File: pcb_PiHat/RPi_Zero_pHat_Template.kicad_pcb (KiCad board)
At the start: 2 copper layers, 65 x 30 mm, 9 parts, among them J1 RPi_GPIO, J2 Isolated_ISP, J3 Isolated_ISP, J4 Conn_Relay, J5 Conn_Relay

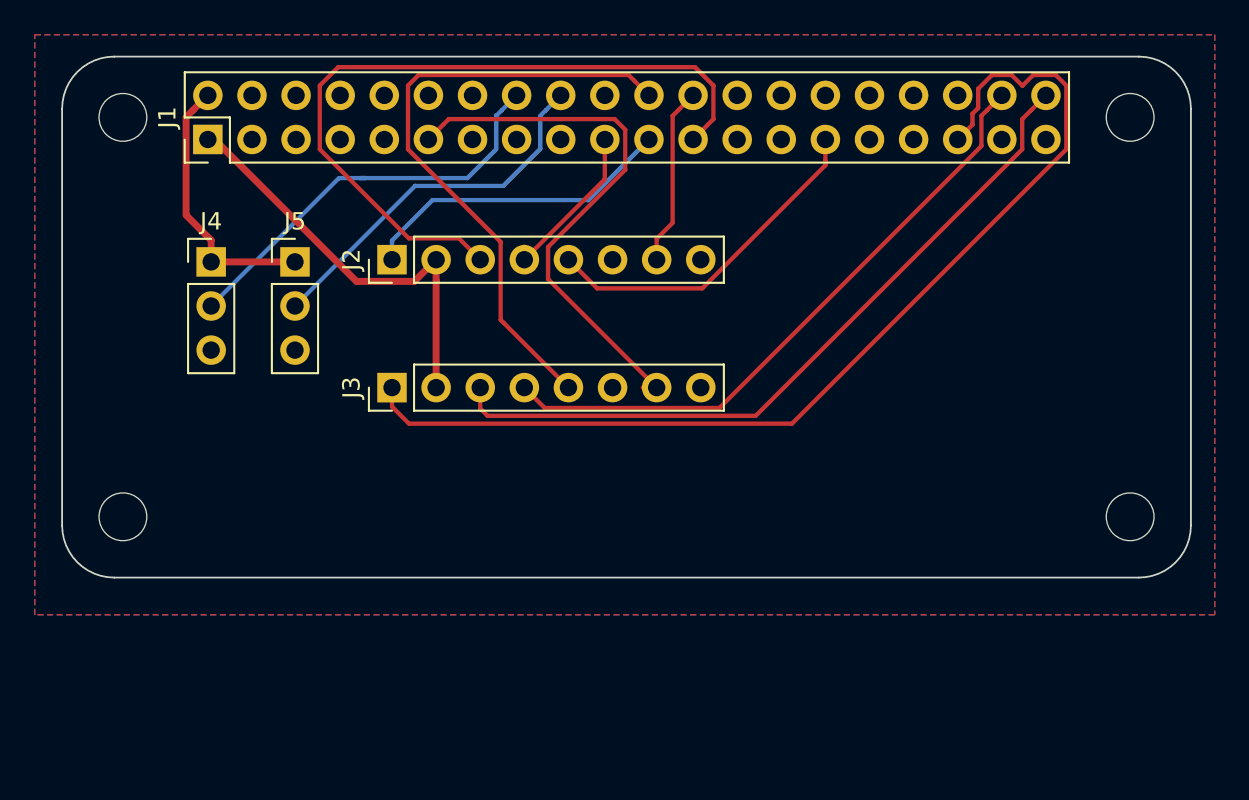
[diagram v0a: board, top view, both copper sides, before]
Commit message: raspi hat toteutettu versio
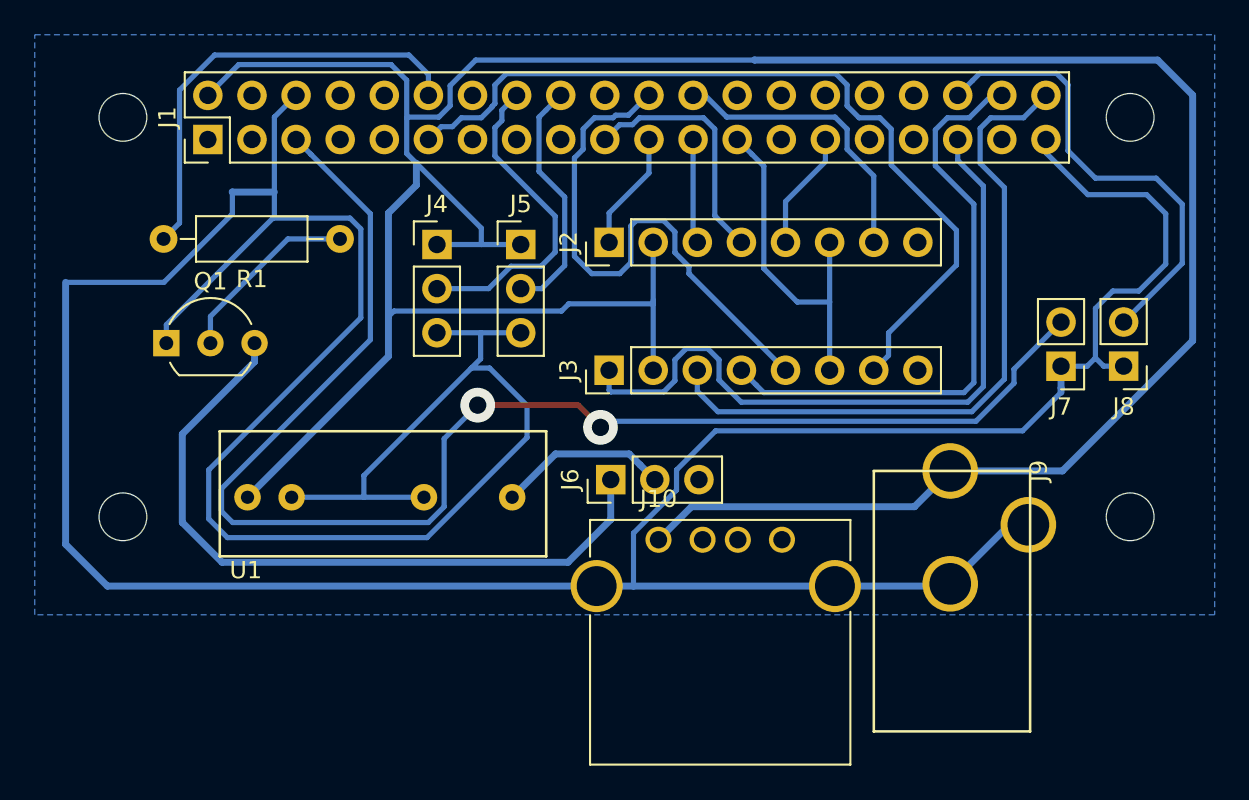
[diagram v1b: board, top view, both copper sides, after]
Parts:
- added J10: USB_A, Connectors:USB_A, F.Cu at (46.8, 52.3)
- added J6: Conn_01x03, Pin_Headers:Pin_Header_Straight_1x03_Pitch2.54mm, F.Cu at (44.1, 48.9)
- added J7: Conn_switch, Pin_Headers:Pin_Header_Straight_1x02_Pitch2.54mm, F.Cu at (70.0, 42.3)
- added J8: Conn_switch, Pin_Headers:Pin_Header_Straight_1x02_Pitch2.54mm, F.Cu at (73.6, 42.3)
- added J9: 5V_in, 5V_power:5V_power, F.Cu at (63.6, 48.4)
- added Q1: Q_NPN_EBC, TO_SOT_Packages_THT:TO-92_Inline_Wide, F.Cu at (18.5, 41.0)
- added R1: R, Resistors_THT:R_Axial_DIN0207_L6.3mm_D2.5mm_P10.16mm_Horizontal, F.Cu at (28.5, 35.0)
- added U1: SPUN02L-12, SPUN02L-12:SPUN02L-12, F.Cu at (23.2, 49.9)
- moved J4 13.0 mm to (34.1, 35.3)
- moved J5 13.0 mm to (38.9, 35.3)
- moved J2 12.5 mm to (44.0, 35.2)
- moved J3 12.5 mm to (44.0, 42.6)
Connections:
- J1 pad 1: +3V3 -> Net-(J1-Pad1)
- J2 pad 2: +3V3 -> Net-(J1-Pad2)
- J3 pad 2: +3V3 -> Net-(J1-Pad2)
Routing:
- net GND: track 0.00 -> 259.9 mm
- net Net-(J1-Pad2): track 15.5 -> 172.6 mm
- net Net-(J1-Pad5): track 0.00 -> 84.0 mm, vias 0 -> 2
- net Net-(J6-Pad1): track 0.00 -> 41.0 mm
- net Net-(J1-Pad23): track 42.7 -> 6.02 mm
- net Net-(J1-Pad36): track 0.00 -> 27.0 mm
- net Net-(J1-Pad12): track 0.00 -> 25.8 mm
- net +3V3: track 24.4 -> 0.00 mm
- net Net-(J1-Pad35): track 60.1 -> 41.7 mm
- net Net-(J1-Pad11): track 32.2 -> 48.3 mm
- net Net-(J1-Pad29): track 19.9 -> 6.87 mm
- net Net-(J1-Pad21): track 18.3 -> 6.87 mm
- net Net-(Q1-Pad2): track 0.00 -> 10.8 mm
- net Net-(J6-Pad2): track 0.00 -> 9.86 mm
- net Net-(J1-Pad18): track 21.4 -> 14.0 mm
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- removed copper zone on F.Cu, net GND
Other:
- board outline removed
- net class Default: clearance 0.2 -> 0.25; trace_width 0.25 -> 0.3; via_dia 0.6 -> 2; via_drill 0.4 -> 1
- rule trace_clearance: 0.2 -> 0.25
